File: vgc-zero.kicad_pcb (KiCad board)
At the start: 2 copper layers, 53 x 87.5 mm, 36 parts, among them J1 Conn_01x06_Pin, J2 Conn_01x06_Pin, J3 Conn_01x06_Pin, SW1 SW_Push, SW10 SW_Push, SW11 SW_SPDT, SW2 SW_Push, SW3 SW_Push, SW4 SW_Push, SW5 SW_Push, SW6 SW_Push, SW7 SW_Push, SW8 SW_Push, SW9 SW_Push

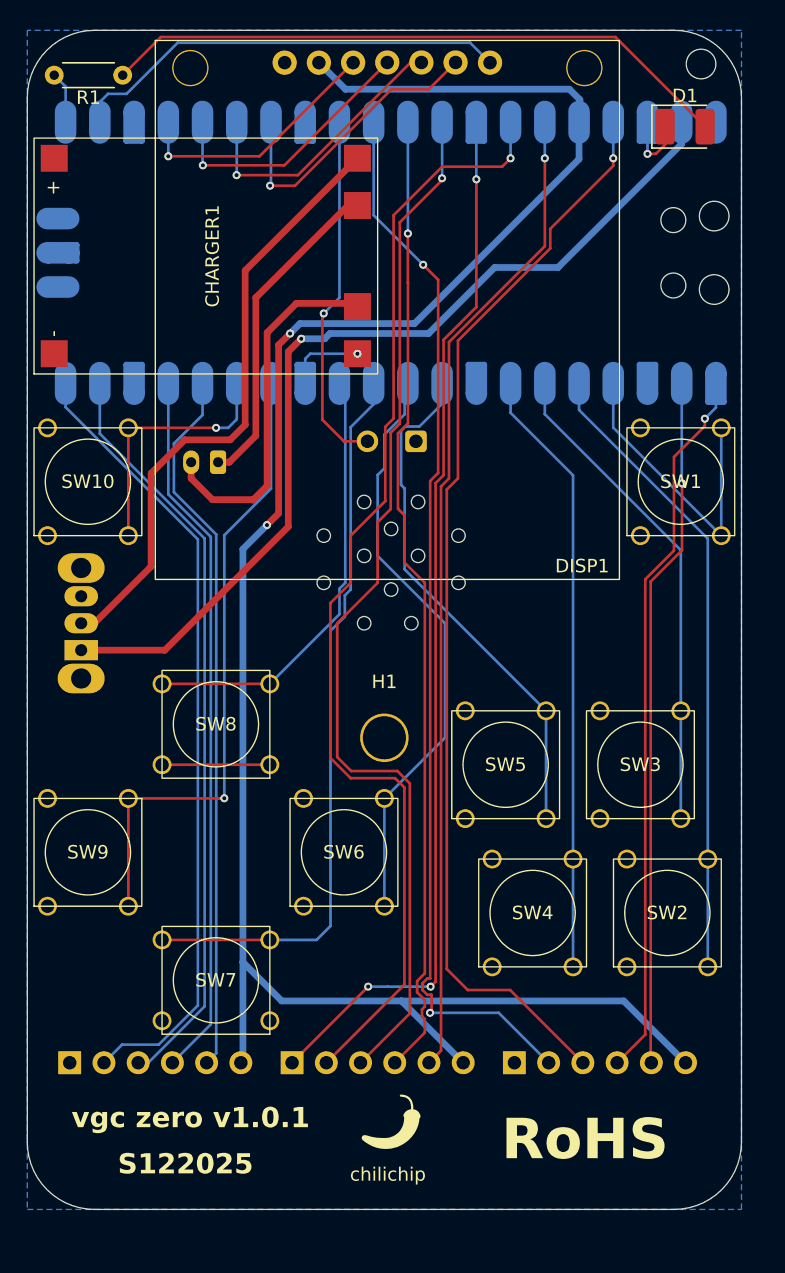
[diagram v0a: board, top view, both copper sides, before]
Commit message: update to 1.1.0
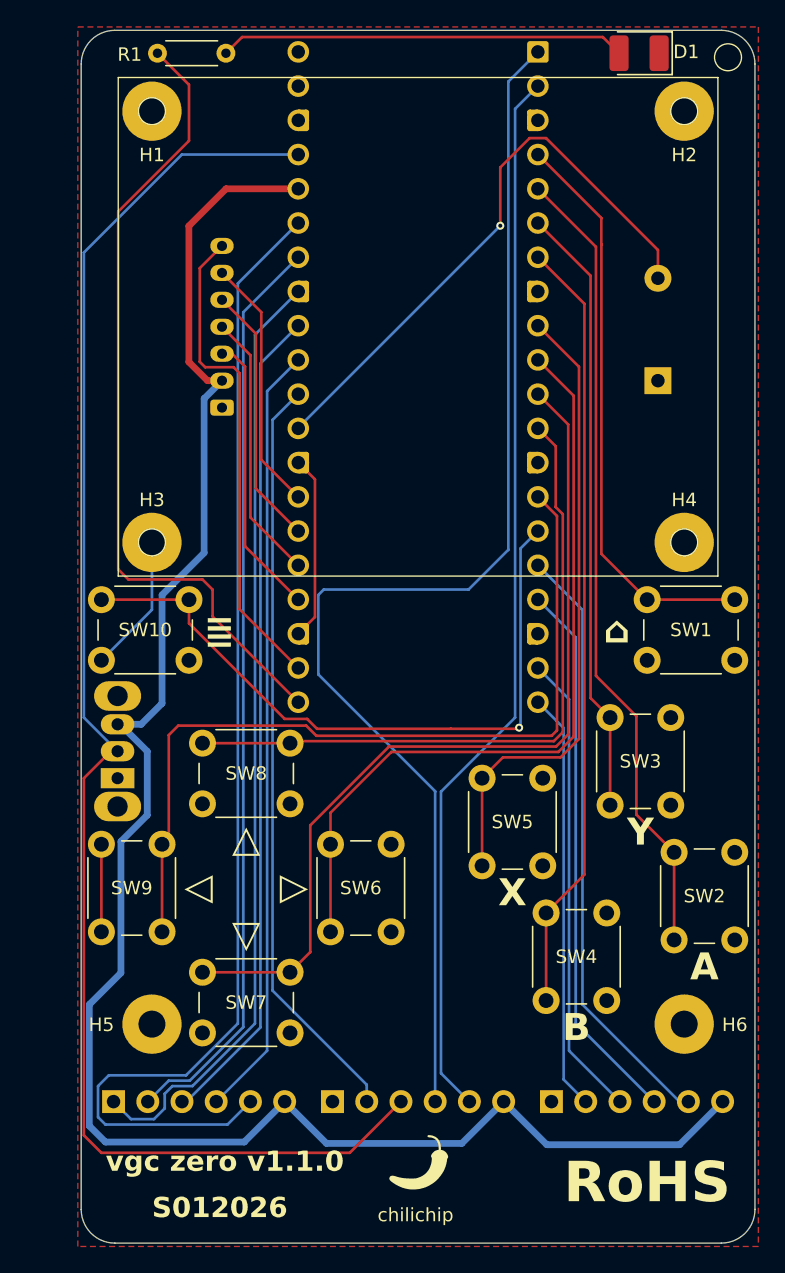
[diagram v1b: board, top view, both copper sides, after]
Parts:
- removed ? (x12): , 
- removed BT1: LIPO-BATTERY, Connector_JST:JST_PH_S2B-PH-K_1x02_P2.00mm_Horizontal
- removed CHARGER1: TP4056_CHARGER, vgc-zero-footprints:Tp4056_Charger
- removed REF**: MountingHole_2.2mm_M2, MountingHole:MountingHole_2.2mm_M2
- added H2: MountingHole_Pad, MountingHole:MountingHole_2.2mm_M2_Pad, F.Cu at (99.2, 44.0)
- added H3: MountingHole_Pad, MountingHole:MountingHole_2.2mm_M2_Pad, F.Cu at (59.8, 76.0)
- added H4: MountingHole_Pad, MountingHole:MountingHole_2.2mm_M2_Pad, F.Cu at (99.2, 76.0)
- added H5: MountingHole_Pad, MountingHole:MountingHole_2.2mm_M2_Pad, F.Cu at (59.8, 111.8)
- added H6: MountingHole_Pad, MountingHole:MountingHole_2.2mm_M2_Pad, F.Cu at (99.2, 111.8)
- DISP1: footprint vgc-zero-footprints:SSD1351_OLED_128x128 -> Connector_JST:JST_PH_S7B-PH-K_1x07_P2.00mm_Horizontal; moved to B.Cu
- H1: footprint MountingHole:MountingHole_3.2mm_M3_Pad -> MountingHole:MountingHole_2.2mm_M2_Pad
- LS1: footprint Connector_Wire:SolderWire-0.1sqmm_1x02_P3.6mm_D0.4mm_OD1mm -> Buzzer_Beeper:Buzzer_12x9.5RM7.6
- MCU1: footprint Module:RaspberryPi_Pico_SMD_HandSolder -> Module:RaspberryPi_Pico_Common_THT
- SW1, SW10, SW2, SW3, SW4, SW5, SW6, SW7, SW8, SW9: footprint vgc-zero-footprints:SW_PUSH_RUBBER_8mm -> Button_Switch_THT:SW_PUSH_6mm_H5mm
- moved H1 49.6 mm to (59.8, 44.0)
- moved J3 35.9 mm to (89.4, 117.5)
- moved DISP1 26.0 mm to (65.0, 66.0), turned to 90 degrees
- moved LS1 18.5 mm to (97.3, 64.0), turned to 90 degrees
- moved MCU1 18.5 mm to (88.4, 39.6), turned to 180 degrees
- moved SW10 14.8 mm to (62.5, 84.8), turned to 180 degrees
- moved J2 13.8 mm to (73.2, 117.5)
- moved J1 13.6 mm to (56.9, 117.5)
- moved SW2 12.4 mm to (103.0, 99.0), turned to -90 degrees
- moved SW1 12.2 mm to (103.0, 84.8), turned to 180 degrees
- moved SW4 10.3 mm to (93.5, 103.5), turned to -90 degrees
- moved SW11 9.88 mm to (57.2, 93.5)
- moved SW3 9.76 mm to (98.2, 89.0), turned to -90 degrees
- moved SW6 8.80 mm to (77.5, 98.4), turned to -90 degrees
- moved R1 7.83 mm to (60.2, 39.7)
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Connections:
- MCU1 pad 39: /VCC -> unconnected-(MCU1-VSYS-Pad39)
- SW11 pad 1: /VCC -> /GND
- SW11 pad 2: Net-(CHARGER1-OUT+) -> Net-(J2-Pin_3)
- SW11 pad 3: unconnected-(SW11-C-Pad3) -> 3V3
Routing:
- net /VCC: track 69.3 -> 0.00 mm, vias 1 -> 0
- net Net-(MCU1-GPIO16): track 3.84 -> 60.1 mm
- net Net-(CHARGER1-OUT+): track 45.5 -> 0.00 mm
- net Net-(J2-Pin_4): track 53.5 -> 94.5 mm, vias 1 -> 0
- net Net-(MCU1-GPIO11): track 19.0 -> 51.2 mm
- net Net-(J2-Pin_3): track 80.9 -> 112.4 mm, vias 1 -> 0
- net Net-(J3-Pin_2): track 59.0 -> 31.1 mm
- net Net-(J2-Pin_5): track 51.4 -> 79.2 mm, vias 1 -> 0
- net Net-(BT1--): track 27.0 -> 0.00 mm
- net Net-(BT1-+): track 24.2 -> 0.00 mm
- net Net-(J2-Pin_2): track 79.5 -> 56.2 mm, vias 2 -> 0
- net Net-(J3-Pin_3): track 56.1 -> 34.7 mm
- net Net-(MCU1-GPIO2): track 22.6 -> 42.9 mm
- net Net-(MCU1-GPIO9): track 32.8 -> 50.4 mm
- net Net-(J1-Pin_3): track 78.8 -> 61.3 mm, vias 1 -> 0
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- added copper zone on F.Cu, net /GND
- removed copper zone on B.Cu, net /GND
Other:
- board size 53 x 87.5 mm -> 50 x 90 mm
- board text added: "A"
- board text added: "B"
- board text added: "S012026"
- board text added: "X"
- board text added: "Y"
- board text added: "vgc zero v1.1.0"
- board text added: "≣"
- board text added: "⌂"
- board text added: "△"
- board text removed: "S122025"
- board text removed: "vgc zero v1.0.1"
